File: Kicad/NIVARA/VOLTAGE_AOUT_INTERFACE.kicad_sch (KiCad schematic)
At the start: 4 parts

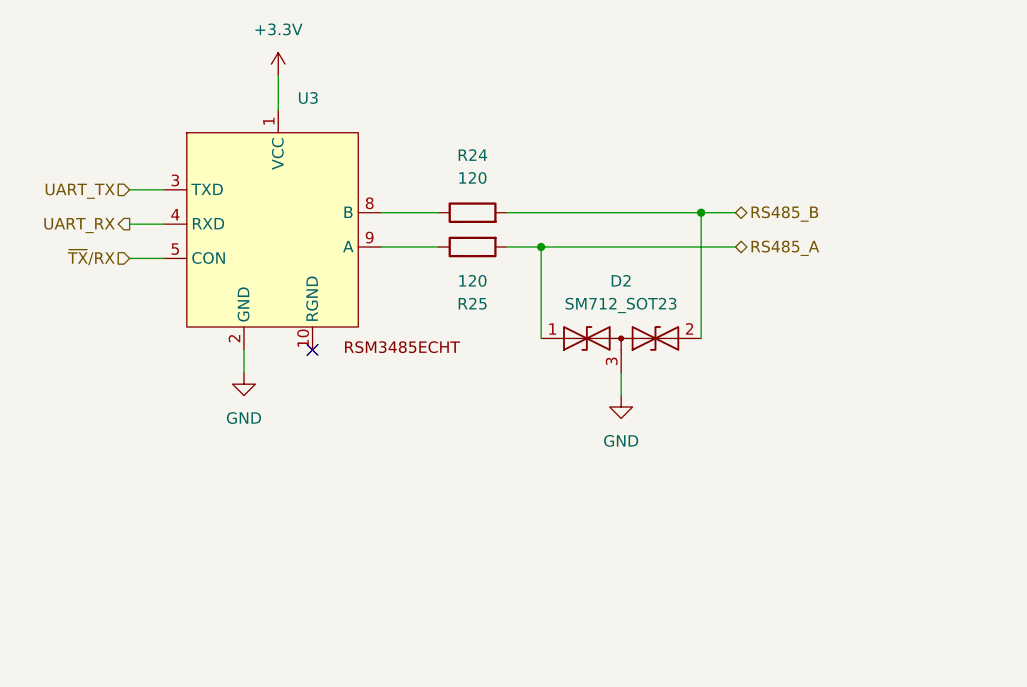
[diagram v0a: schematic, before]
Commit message: .
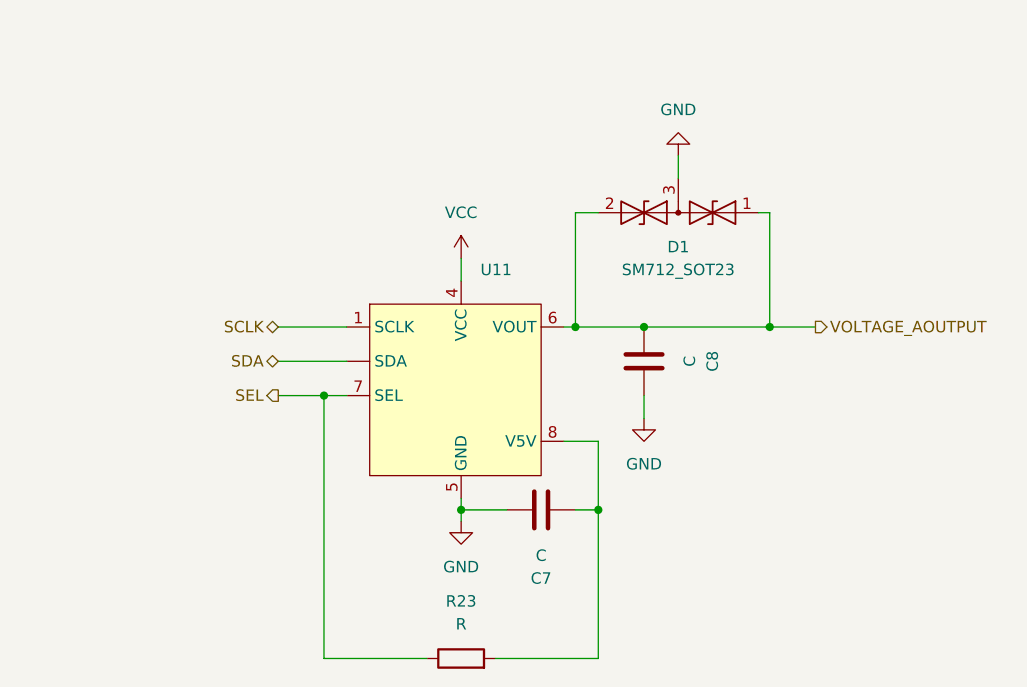
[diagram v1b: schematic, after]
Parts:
- removed D2: SM712_SOT23, Package_TO_SOT_SMD:SOT-23, symbol Diode:SM712_SOT23
- removed R24, R25: 120, symbol Device:R
- removed U3: ~, Riqi_Parts:YLPTEC RSM3485ECHT, symbol Riqi_Parts:YLPTEC_RSM3485ECHT
- added C7, C8: C, symbol Device:C
- added D1: SM712_SOT23, Package_TO_SOT_SMD:SOT-23, symbol Diode:SM712_SOT23
- added R23: R, symbol Device:R
- added U11: ~, Riqi_Parts:eSOP-8, symbol Riqi_Parts:GP8201S
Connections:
- net GND: now also C7.1, C8.1, D1.3 (common), U11.5 (GND)
- new net: C7.2, R23.2, U11.8 (V5V)
- new net SCLK: U11.1 (SCLK)
- new net SDA: U11. (SDA)
- new net SEL: R23.1, U11.7 (SEL)
- new net VCC: U11.4 (VCC)
- new net VOLTAGE_AOUTPUT: C8.2, D1.1 (A1), D1.2 (A2), U11.6 (VOUT)
- no-connect marks 1 -> 0
